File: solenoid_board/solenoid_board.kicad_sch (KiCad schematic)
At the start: 0 parts

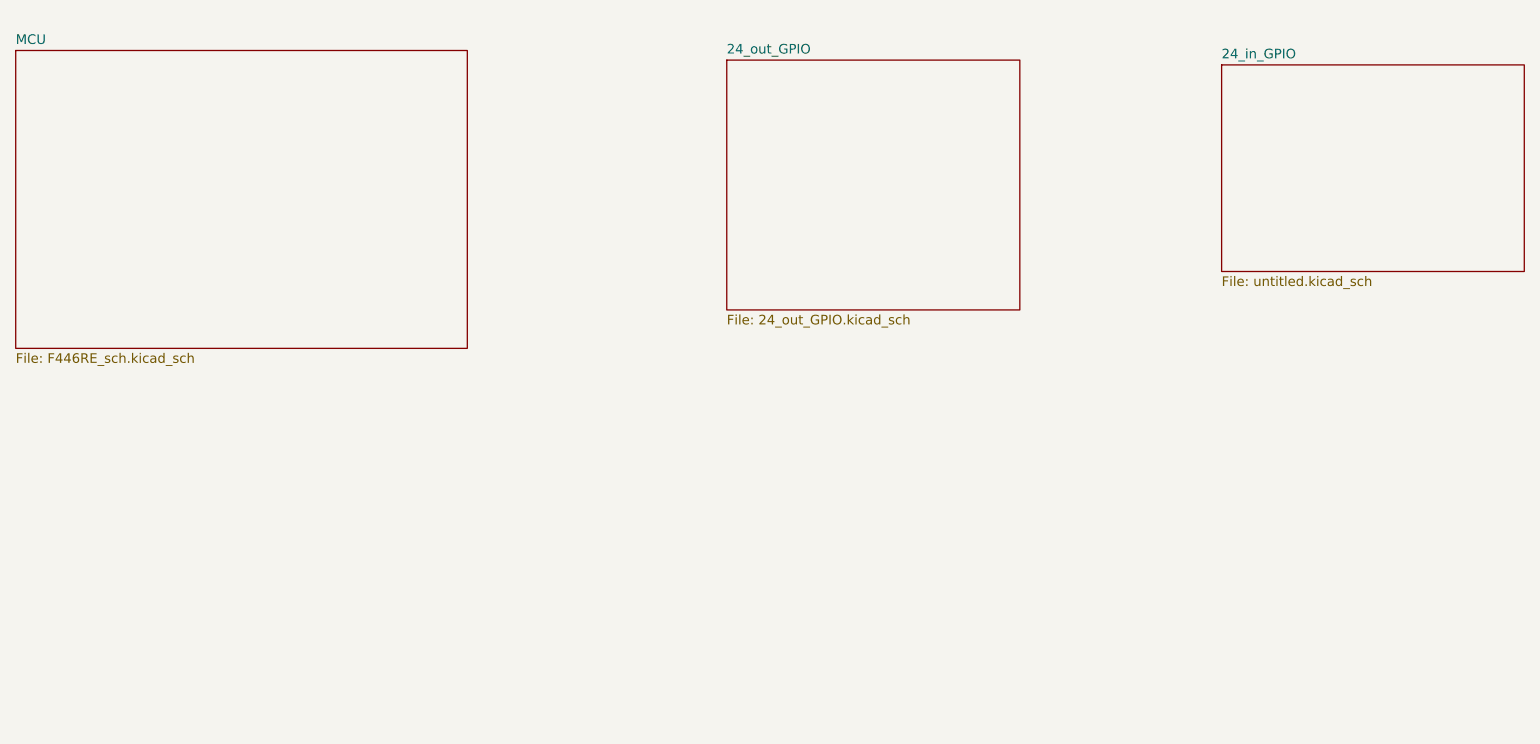
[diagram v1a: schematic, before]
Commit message: solenoid board
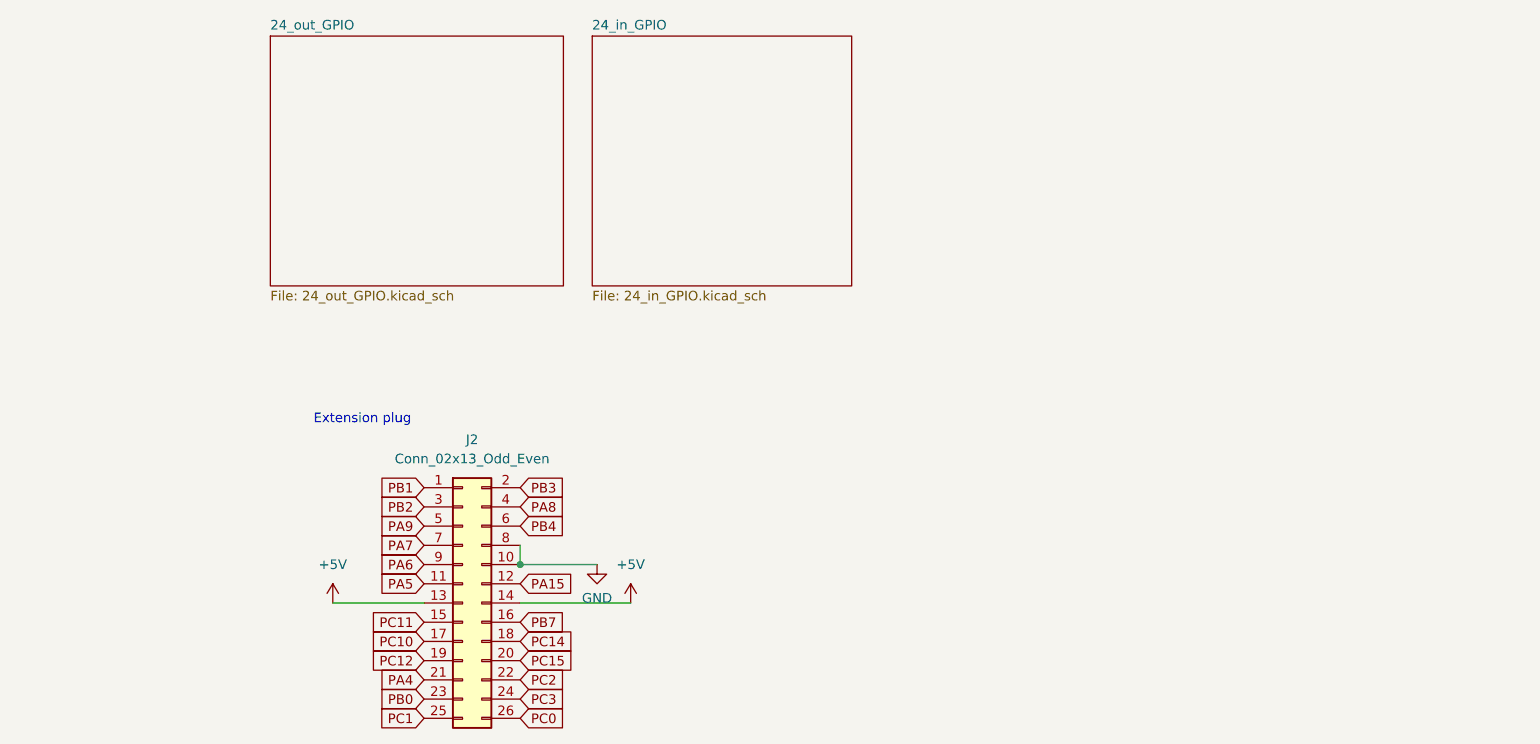
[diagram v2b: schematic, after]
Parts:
- added J2: Conn_02x13_Odd_Even, Connector_IDC:IDC-Header_2x13_P2.54mm_Vertical, symbol Connector_Generic:Conn_02x13_Odd_Even
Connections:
- new net +5V: J2.13 (Pin_13), J2.14 (Pin_14)
- new net GND: J2.10 (Pin_10), J2.8 (Pin_8)
- new net PA15: J2.12 (Pin_12)
- new net PA4: J2.21 (Pin_21)
- new net PA5: J2.11 (Pin_11)
- new net PA6: J2.9 (Pin_9)
- new net PA7: J2.7 (Pin_7)
- new net PA8: J2.4 (Pin_4)
- new net PA9: J2.5 (Pin_5)
- new net PB0: J2.23 (Pin_23)
- new net PB1: J2.1 (Pin_1)
- new net PB2: J2.3 (Pin_3)
- new net PB3: J2.2 (Pin_2)
- new net PB4: J2.6 (Pin_6)
- new net PB7: J2.16 (Pin_16)
- new net PC0: J2.26 (Pin_26)
- new net PC1: J2.25 (Pin_25)
- new net PC10: J2.17 (Pin_17)
- new net PC11: J2.15 (Pin_15)
- new net PC12: J2.19 (Pin_19)
- new net PC14: J2.18 (Pin_18)
- new net PC15: J2.20 (Pin_20)
- new net PC2: J2.22 (Pin_22)
- new net PC3: J2.24 (Pin_24)
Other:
- removed sheet MCU
- sheet 24_in_GPIO: file untitled.kicad_sch -> 24_in_GPIO.kicad_sch
- note added: "Extension plug"
